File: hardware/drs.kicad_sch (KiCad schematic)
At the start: 0 parts

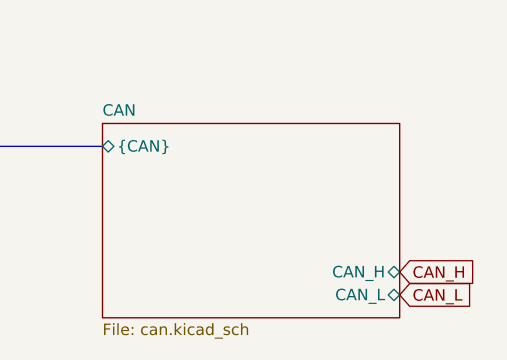
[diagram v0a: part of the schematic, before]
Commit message: pcb update
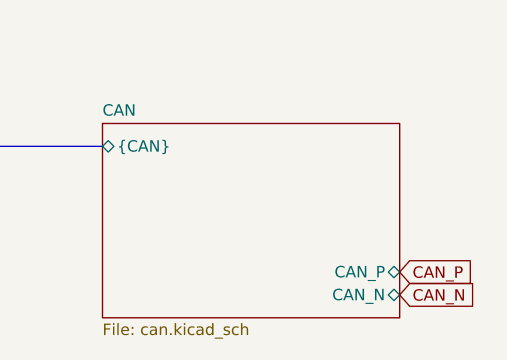
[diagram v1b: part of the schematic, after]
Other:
- sheet CAN ports: added CAN_N, CAN_P; removed CAN_H, CAN_L
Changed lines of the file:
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@@
 		)
 	)
-	(global_label "CAN_H"
+	(global_label "CAN_P"
 		(shape input)
 		(at 236.22 120.65 0)
@@
 		)
 		(property "Intersheetrefs" "${INTERSHEET_REFS}"
-			(at 245.1924 120.65 0)
+			(at 245.1319 120.65 0)
 			(effects
 				(font
@@
 		)
 	)
-	(global_label "CAN_L"
+	(global_label "CAN_N"
 		(shape input)
 		(at 236.22 123.19 0)
@@
 		)
 		(property "Intersheetrefs" "${INTERSHEET_REFS}"
-			(at 244.89 123.19 0)
+			(at 245.1924 123.19 0)
 			(effects
 				(font
@@
 			)
 		)
-		(pin "CAN_H" bidirectional
+		(pin "CAN_P" bidirectional
 			(at 236.22 120.65 0)
 			(effects
@@
 			)
 		)
-		(pin "CAN_L" bidirectional
+		(pin "CAN_N" bidirectional
 			(at 236.22 123.19 0)
 			(effects
